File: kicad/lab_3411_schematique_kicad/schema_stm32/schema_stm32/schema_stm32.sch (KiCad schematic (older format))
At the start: 10 parts

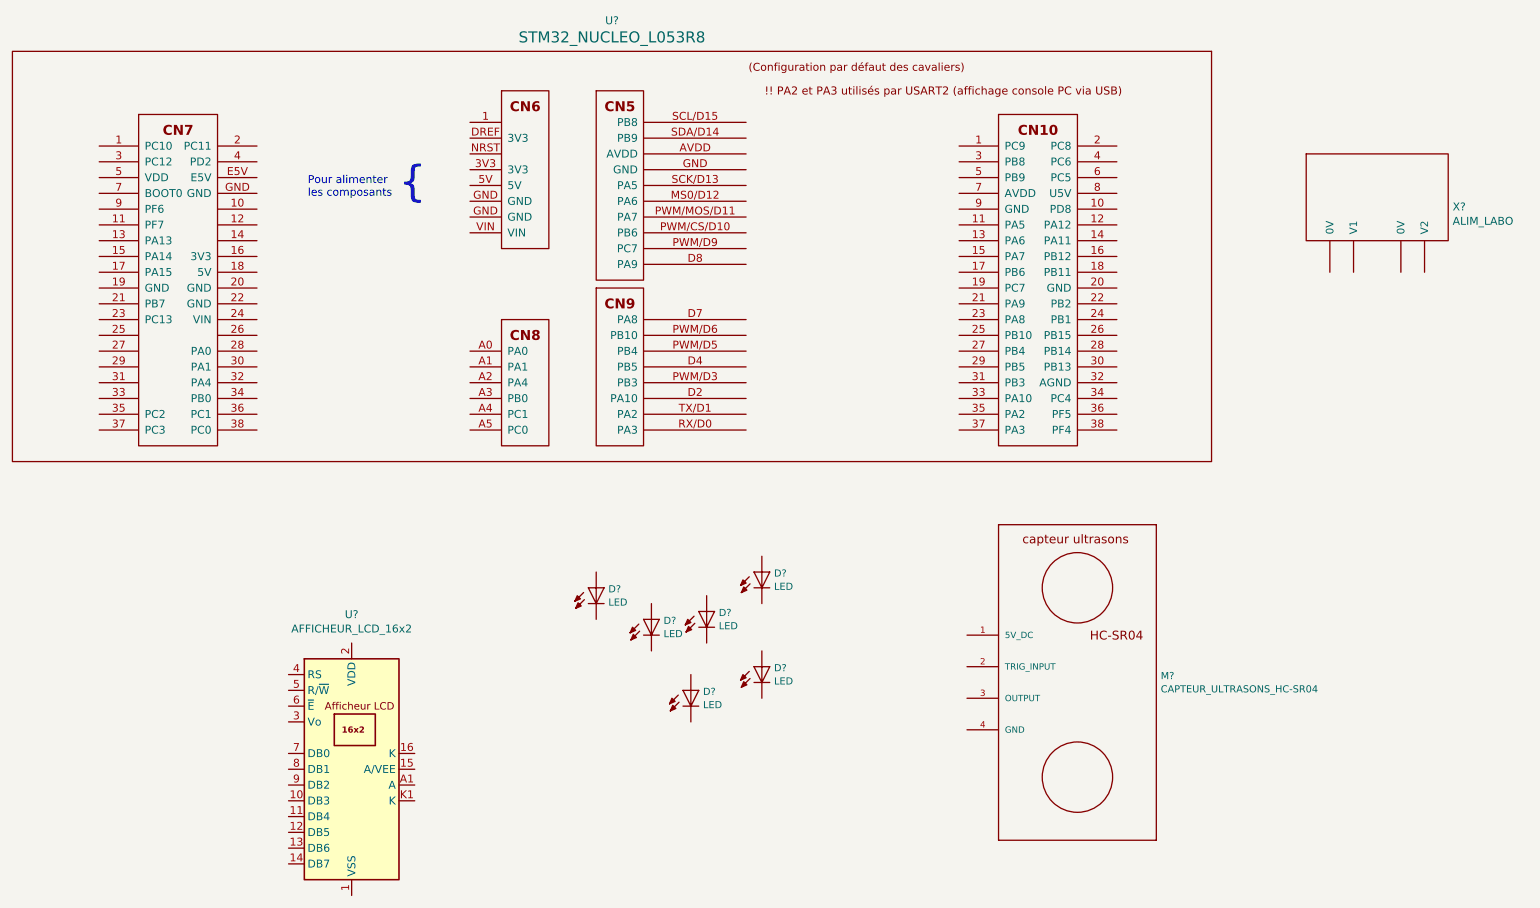
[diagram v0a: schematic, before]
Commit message: Avancement
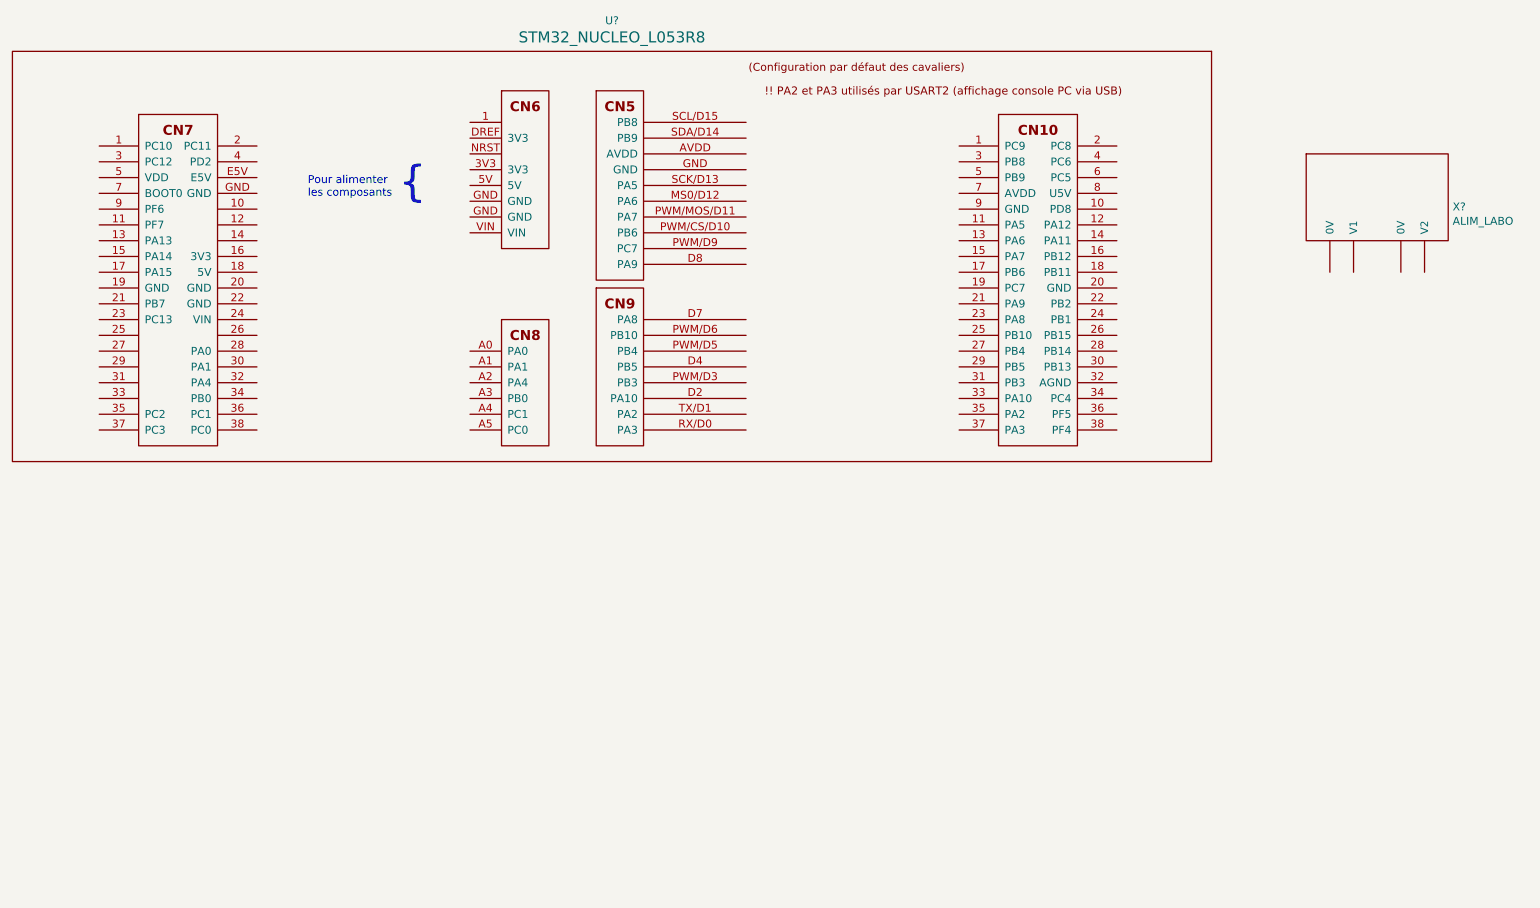
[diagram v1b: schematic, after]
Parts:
- removed D? (x6): LED, lib_esiea_U57X32, symbol lib_esiea:LED
- removed M?: CAPTEUR_ULTRASONS_HC-SR04, HC-SR04, symbol lib_esiea:CAPTEUR_ULTRASONS_HC-SR04
- removed U?: AFFICHEUR_LCD_16x2, Display:RC1602A, symbol lib_esiea:AFFICHEUR_LCD_16x2
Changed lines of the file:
@@
 EESchema Schematic File Version 4
 LIBS:schema_stm32-cache
-EELAYER 29 0
+EELAYER 26 0
 EELAYER END
 $Descr A4 11693 8268
@@
 Text Notes 3072 2031 0    50   ~ 0
 Pour alimenter \nles composants
-$Comp
-L lib_esiea:AFFICHEUR_LCD_16x2 U?
-U 1 1 5CCDD7D9
-P 3350 5650
-F 0 "U?" H 3350 6631 50  0000 C CNN
-F 1 "AFFICHEUR_LCD_16x2" H 3350 6540 50  0000 C CNN
-F 2 "Display:RC1602A" H 3350 4750 50  0001 C CIN
-F 3 "http://www.raystar-optronics.com/down.php?ProID=18" H 2850 6350 50  0001 C CNN
-	1    3350 5650
-	1    0    0    -1
-$EndComp
-$Comp
-L lib_esiea:CAPTEUR_ULTRASONS_HC-SR04 M?
-U 1 1 5CCDE754
-P 7750 4200
-F 0 "M?" H 8478 3342 45  0000 L CNN
-F 1 "CAPTEUR_ULTRASONS_HC-SR04" H 8478 3258 45  0000 L CNN
-F 2 "HC-SR04" H 7780 4350 20  0001 C CNN
-F 3 "" H 7750 4200 50  0001 C CNN
-	1    7750 4200
-	1    0    0    -1
-$EndComp
-$Comp
-L lib_esiea:LED D?
-U 1 1 5CCDF1FB
-P 5600 4650
-F 0 "D?" H 5677 4642 45  0000 L CNN
-F 1 "LED" H 5677 4558 45  0000 L CNN
-F 2 "lib_esiea_U57X32" H 5630 4800 20  0001 C CNN
-F 3 "" H 5600 4650 50  0001 C CNN
-	1    5600 4650
-	1    0    0    -1
-$EndComp
-$Comp
-L lib_esiea:LED D?
-U 1 1 5CCDFBAE
-P 5250 4700
-F 0 "D?" H 5327 4692 45  0000 L CNN
-F 1 "LED" H 5327 4608 45  0000 L CNN
-F 2 "lib_esiea_U57X32" H 5280 4850 20  0001 C CNN
-F 3 "" H 5250 4700 50  0001 C CNN
-	1    5250 4700
-	1    0    0    -1
-$EndComp
-$Comp
-L lib_esiea:LED D?
-U 1 1 5CCE0E59
-P 4900 4500
-F 0 "D?" H 4977 4492 45  0000 L CNN
-F 1 "LED" H 4977 4408 45  0000 L CNN
-F 2 "lib_esiea_U57X32" H 4930 4650 20  0001 C CNN
-F 3 "" H 4900 4500 50  0001 C CNN
-	1    4900 4500
-	1    0    0    -1
-$EndComp
-$Comp
-L lib_esiea:LED D?
-U 1 1 5CCE144D
-P 5950 4400
-F 0 "D?" H 6027 4392 45  0000 L CNN
-F 1 "LED" H 6027 4308 45  0000 L CNN
-F 2 "lib_esiea_U57X32" H 5980 4550 20  0001 C CNN
-F 3 "" H 5950 4400 50  0001 C CNN
-	1    5950 4400
-	1    0    0    -1
-$EndComp
-$Comp
-L lib_esiea:LED D?
-U 1 1 5CCE1A93
-P 5500 5150
-F 0 "D?" H 5577 5142 45  0000 L CNN
-F 1 "LED" H 5577 5058 45  0000 L CNN
-F 2 "lib_esiea_U57X32" H 5530 5300 20  0001 C CNN
-F 3 "" H 5500 5150 50  0001 C CNN
-	1    5500 5150
-	1    0    0    -1
-$EndComp
-$Comp
-L lib_esiea:LED D?
-U 1 1 5CCE1DD7
-P 5950 5000
-F 0 "D?" H 6027 4992 45  0000 L CNN
-F 1 "LED" H 6027 4908 45  0000 L CNN
-F 2 "lib_esiea_U57X32" H 5980 5150 20  0001 C CNN
-F 3 "" H 5950 5000 50  0001 C CNN
-	1    5950 5000
-	1    0    0    -1
-$EndComp
 $EndSCHEMATC

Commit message: MAJ Kicad
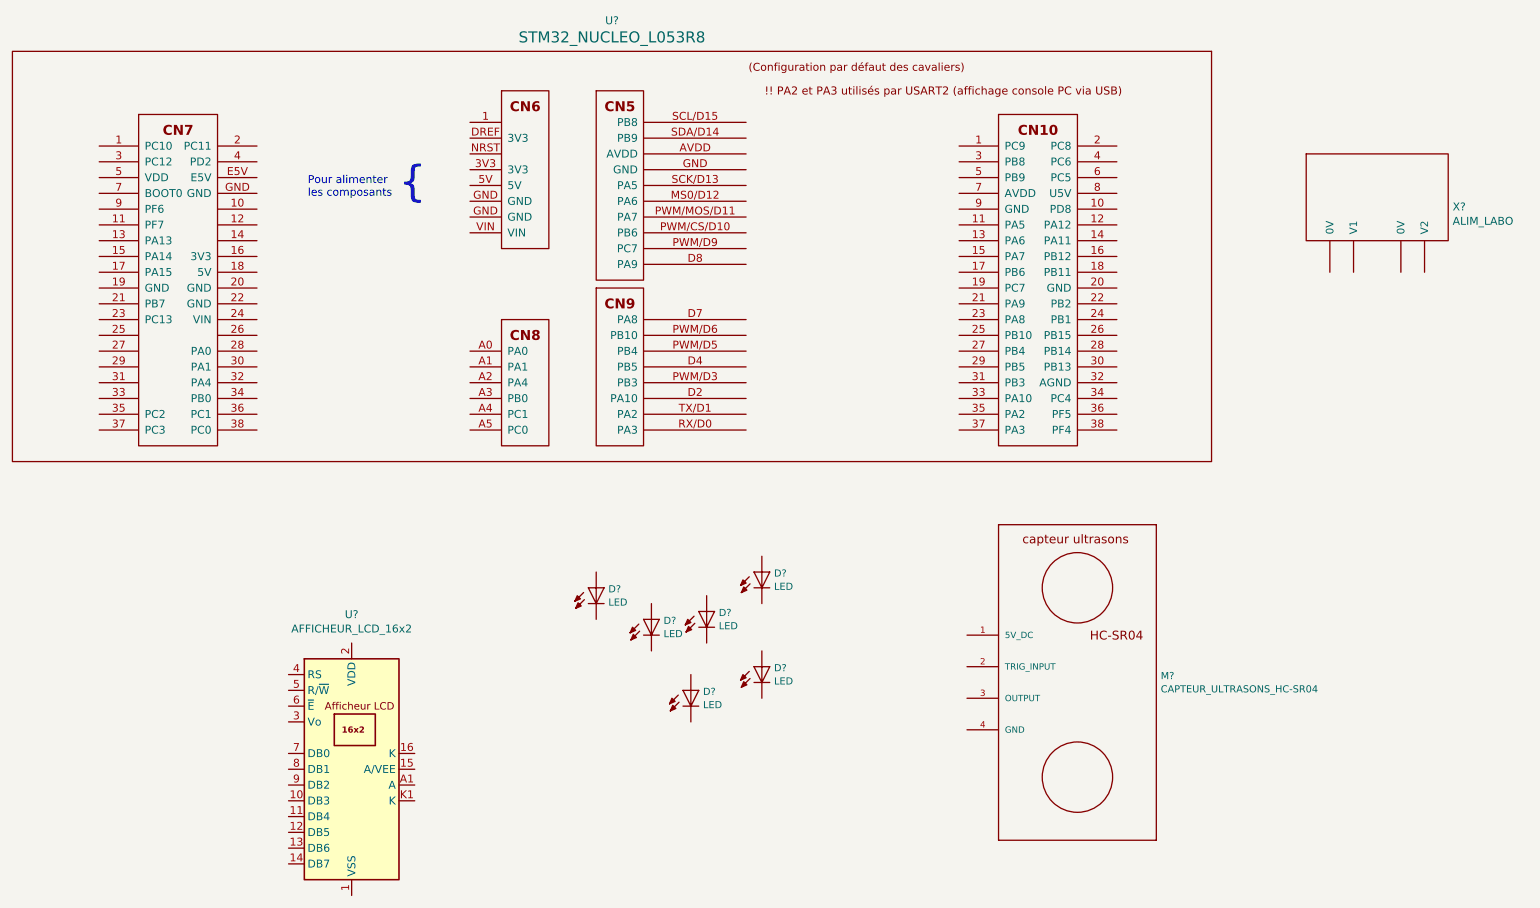
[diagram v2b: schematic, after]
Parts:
- added D? (x6): LED, lib_esiea_U57X32, symbol lib_esiea:LED
- added M?: CAPTEUR_ULTRASONS_HC-SR04, HC-SR04, symbol lib_esiea:CAPTEUR_ULTRASONS_HC-SR04
- added U?: AFFICHEUR_LCD_16x2, Display:RC1602A, symbol lib_esiea:AFFICHEUR_LCD_16x2
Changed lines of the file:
@@
 EESchema Schematic File Version 4
 LIBS:schema_stm32-cache
-EELAYER 26 0
+EELAYER 29 0
 EELAYER END
 $Descr A4 11693 8268
@@
 Text Notes 3072 2031 0    50   ~ 0
 Pour alimenter \nles composants
+$Comp
+L lib_esiea:AFFICHEUR_LCD_16x2 U?
+U 1 1 5CCDD7D9
+P 3350 5650
+F 0 "U?" H 3350 6631 50  0000 C CNN
+F 1 "AFFICHEUR_LCD_16x2" H 3350 6540 50  0000 C CNN
+F 2 "Display:RC1602A" H 3350 4750 50  0001 C CIN
+F 3 "http://www.raystar-optronics.com/down.php?ProID=18" H 2850 6350 50  0001 C CNN
+	1    3350 5650
+	1    0    0    -1
+$EndComp
+$Comp
+L lib_esiea:CAPTEUR_ULTRASONS_HC-SR04 M?
+U 1 1 5CCDE754
+P 7750 4200
+F 0 "M?" H 8478 3342 45  0000 L CNN
+F 1 "CAPTEUR_ULTRASONS_HC-SR04" H 8478 3258 45  0000 L CNN
+F 2 "HC-SR04" H 7780 4350 20  0001 C CNN
+F 3 "" H 7750 4200 50  0001 C CNN
+	1    7750 4200
+	1    0    0    -1
+$EndComp
+$Comp
+L lib_esiea:LED D?
+U 1 1 5CCDF1FB
+P 5600 4650
+F 0 "D?" H 5677 4642 45  0000 L CNN
+F 1 "LED" H 5677 4558 45  0000 L CNN
+F 2 "lib_esiea_U57X32" H 5630 4800 20  0001 C CNN
+F 3 "" H 5600 4650 50  0001 C CNN
+	1    5600 4650
+	1    0    0    -1
+$EndComp
+$Comp
+L lib_esiea:LED D?
+U 1 1 5CCDFBAE
+P 5250 4700
+F 0 "D?" H 5327 4692 45  0000 L CNN
+F 1 "LED" H 5327 4608 45  0000 L CNN
+F 2 "lib_esiea_U57X32" H 5280 4850 20  0001 C CNN
+F 3 "" H 5250 4700 50  0001 C CNN
+	1    5250 4700
+	1    0    0    -1
+$EndComp
+$Comp
+L lib_esiea:LED D?
+U 1 1 5CCE0E59
+P 4900 4500
+F 0 "D?" H 4977 4492 45  0000 L CNN
+F 1 "LED" H 4977 4408 45  0000 L CNN
+F 2 "lib_esiea_U57X32" H 4930 4650 20  0001 C CNN
+F 3 "" H 4900 4500 50  0001 C CNN
+	1    4900 4500
+	1    0    0    -1
+$EndComp
+$Comp
+L lib_esiea:LED D?
+U 1 1 5CCE144D
+P 5950 4400
+F 0 "D?" H 6027 4392 45  0000 L CNN
+F 1 "LED" H 6027 4308 45  0000 L CNN
+F 2 "lib_esiea_U57X32" H 5980 4550 20  0001 C CNN
+F 3 "" H 5950 4400 50  0001 C CNN
+	1    5950 4400
+	1    0    0    -1
+$EndComp
+$Comp
+L lib_esiea:LED D?
+U 1 1 5CCE1A93
+P 5500 5150
+F 0 "D?" H 5577 5142 45  0000 L CNN
+F 1 "LED" H 5577 5058 45  0000 L CNN
+F 2 "lib_esiea_U57X32" H 5530 5300 20  0001 C CNN
+F 3 "" H 5500 5150 50  0001 C CNN
+	1    5500 5150
+	1    0    0    -1
+$EndComp
+$Comp
+L lib_esiea:LED D?
+U 1 1 5CCE1DD7
+P 5950 5000
+F 0 "D?" H 6027 4992 45  0000 L CNN
+F 1 "LED" H 6027 4908 45  0000 L CNN
+F 2 "lib_esiea_U57X32" H 5980 5150 20  0001 C CNN
+F 3 "" H 5950 5000 50  0001 C CNN
+	1    5950 5000
+	1    0    0    -1
+$EndComp
 $EndSCHEMATC
